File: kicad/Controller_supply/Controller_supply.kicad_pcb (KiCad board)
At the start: 2 copper layers, 8 parts, among them J1 Conn_01x03_Pin, U1 MC7824, U2 MC7924

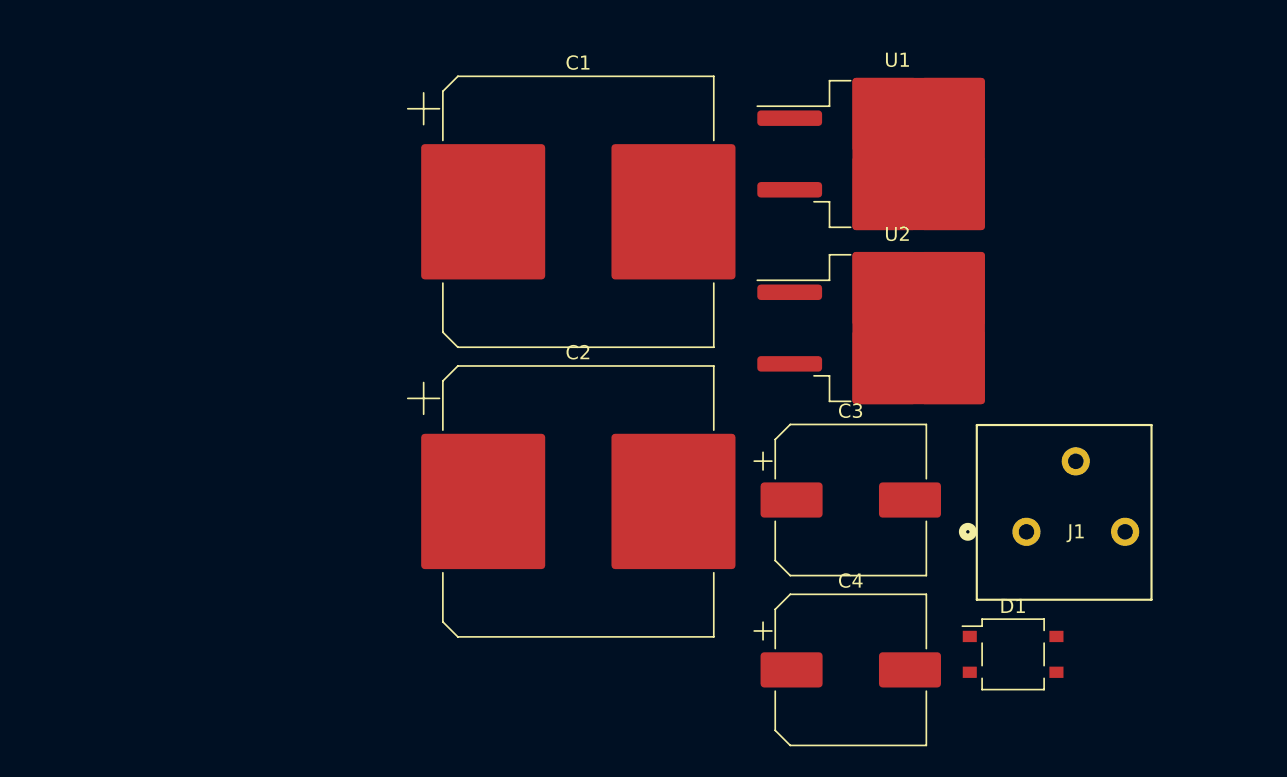
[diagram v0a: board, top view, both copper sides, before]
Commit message: Updated internal power supply board and rear board.Please
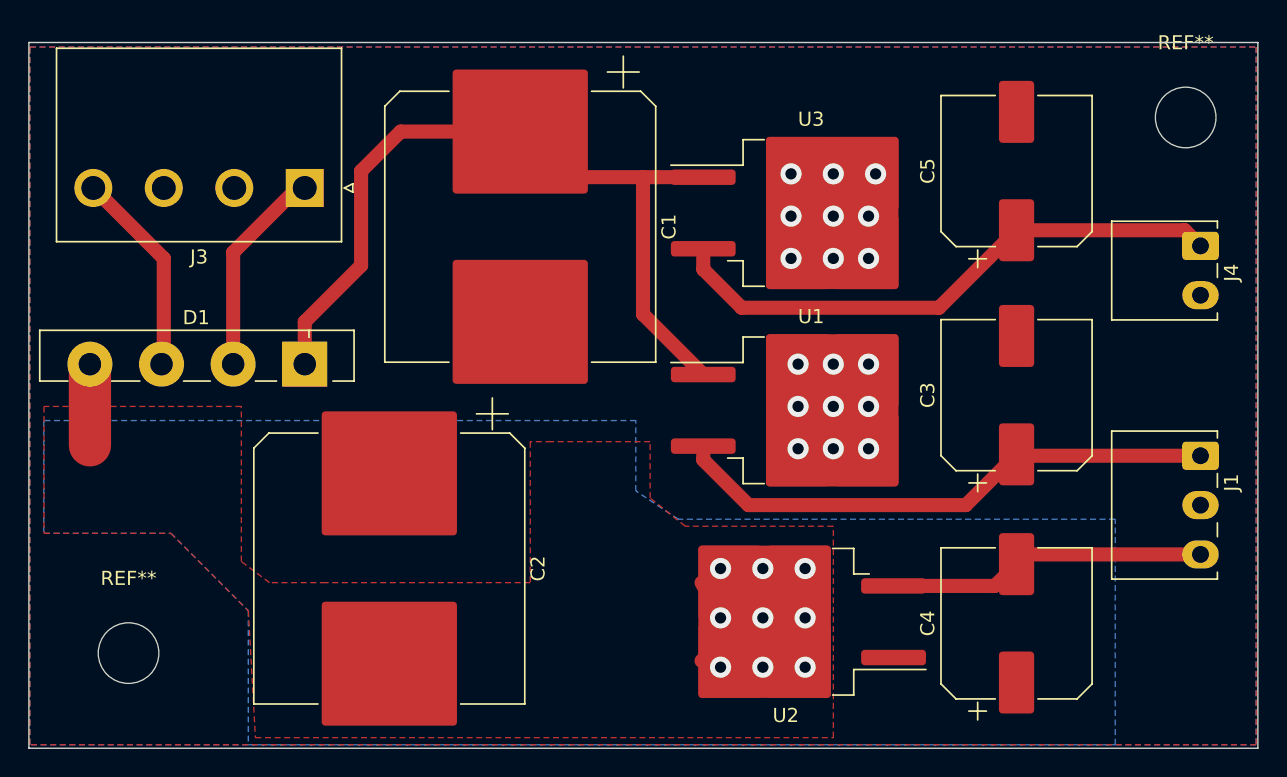
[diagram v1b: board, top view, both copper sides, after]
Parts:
- added C5: 220uF, Capacitor_SMD:CP_Elec_10x10.5, F.Cu at (152.0, 64.8)
- added J3: Conn_01x04_Pin, Connector_THT:Generic_pin-to-housing_1x04_P5.00mm_Horizontal, F.Cu at (101.5, 66.0)
- added J4: Conn_01x02, Connector_THT:Generic_7x7.5mm-footprt_1x02_P3.50mm_Horizontal, F.Cu at (165.1, 70.1)
- added REF**: MountingHole_4.3mm_M4, MountingHole:MountingHole_4.3mm_M4, F.Cu at (164.0, 61.0)
- added REF**: MountingHole_4.3mm_M4, MountingHole:MountingHole_4.3mm_M4, F.Cu at (89.0, 99.0)
- added U3: MC7824, Package_TO_SOT_SMD:TO-263-2, F.Cu at (137.4, 67.8)
- D1: value CDBHD1100L-G -> GBU4A; footprint Package_TO_SOT_SMD:TO-269AA -> Diode_THT:Diode_Bridge_Vishay_GBU
- J1: footprint Connector_THT:CONN_1985205 -> Connector_THT:Generic_10.5x7.5mm-footprt_1x03_P3.50mm_Horizontal
- moved D1 54.3 mm to (101.5, 78.5), turned to 180 degrees
- moved U2 22.3 mm to (135.6, 96.8), turned to 180 degrees
- moved U1 19.2 mm to (137.4, 81.8)
- moved C2 14.2 mm to (107.5, 93.0), turned to -90 degrees
- moved C3 13.9 mm to (152.0, 80.7), turned to 90 degrees
- moved C4 12.2 mm to (152.0, 96.9), turned to 90 degrees
- moved J1 8.84 mm to (165.1, 85.0), turned to -90 degrees
- moved C1 4.25 mm to (116.8, 68.8), turned to -90 degrees
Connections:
- C2 pad 2: Net-(D1--) -> Net-(U2-VI)
- D1 pad 2: Net-(D1--) -> -24AC
- D1 pad 3: -24AC -> +24AC
- D1 pad 4: +24AC -> Net-(U2-VI)
- J1 pad 1: Line Hot -> +24VDC
- J1 pad 3: Line Neutral -> -24VDC
- U2 pad 2: Net-(D1--) -> Net-(U2-VI)
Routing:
- net Net-(D1-+): track 0.00 -> 57.9 mm
- net +24VDC_fan: track 0.00 -> 40.6 mm
- net +24VDC: track 0.00 -> 39.1 mm
- net Net-(U2-VI): track 0.00 -> 27.9 mm, vias 0 -> 9
- net -24VDC: track 0.00 -> 22.7 mm
- net -24AC: track 0.00 -> 14.9 mm
- net +24AC: track 0.00 -> 14.6 mm
- net GND: vias 0 -> 18
- added copper zone on B.Cu, net GND
- added copper zone on F.Cu, net GND
- added copper zone on B.Cu, net Net-(U2-VI)
- added copper zone on F.Cu, net Net-(U2-VI)
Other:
- board outline added: 87.2 x 50.1 mm
